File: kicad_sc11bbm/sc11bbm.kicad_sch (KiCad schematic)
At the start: 17 parts, among them M1 Brushless motor Right, M2 Brushless motor Left, Q1 2SK4017, U1 ESC_R, U2 ESC_L, U3 L3GD20H, U4 QMC5883L, U5 BMP280, U6 MW-R-DP-W, U7 AE-GYSFDMAXB, U8 ADXL335, U9 SD_CARD_DIP

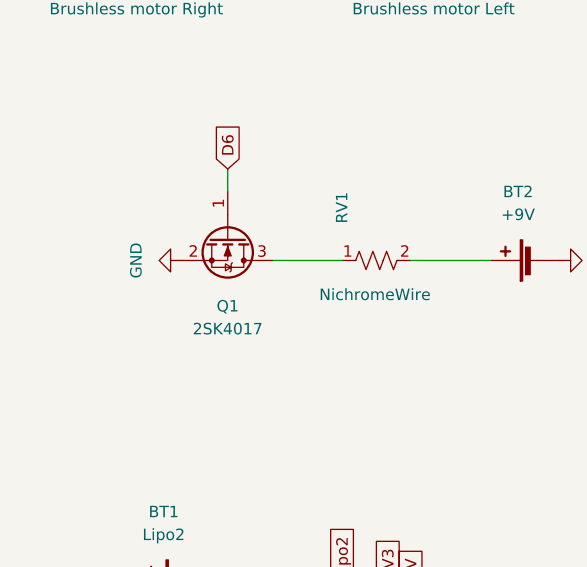
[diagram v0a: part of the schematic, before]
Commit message: Order completed for Board ver1.0
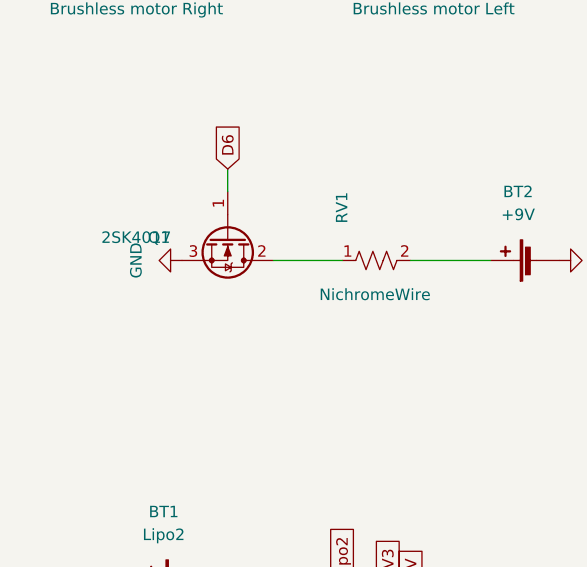
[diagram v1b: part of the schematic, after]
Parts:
- U3: footprint (none) -> sc11bbm:L3GD20H
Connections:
- net GND: now also Q1.3 (S); no longer Q1.2 (S)
- net at RV1.1: now also Q1.2 (D); no longer Q1.3 (D)
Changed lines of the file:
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@@
   (symbol (lib_id "Transistor_FET:2N7002E") (at 66.04 85.09 270) (unit 1)
     (in_bom yes) (on_board yes) (fields_autoplaced)
-    (property "Reference" "Q1" (id 0) (at 66.04 92.71 90))
-    (property "Value" "2SK4017" (id 1) (at 66.04 95.25 90))
-    (property "Footprint" "sc11bbm:2SK4017" (id 2) (at 64.135 90.17 0)
+    (property "Reference" "Q1" (id 0) (at 58.42 85.09 90))
+    (property "Value" "2SK4017" (id 1) (at 55.88 85.09 90))
+    (property "Footprint" "sc11bbm:2SK4017" (id 2) (at 60.96 83.185 0)
       (effects (font (size 1.27 1.27) italic) (justify left) hide)
     )
@@
     (property "Reference" "U3" (id 0) (at 199.39 111.76 0))
     (property "Value" "L3GD20H" (id 1) (at 199.39 114.3 0))
-    (property "Footprint" "" (id 2) (at 199.39 114.3 0)
+    (property "Footprint" "sc11bbm:L3GD20H" (id 2) (at 199.39 114.3 0)
       (effects (font (size 1.27 1.27)) hide)
     )
@@
     )
     (path "/bce30d9d-5959-43c2-901a-216240c51ddc"
-      (reference "U3") (unit 1) (value "L3GD20H") (footprint "")
+      (reference "U3") (unit 1) (value "L3GD20H") (footprint "sc11bbm:L3GD20H")
     )
     (path "/40d8ad8c-b3b9-4b74-ac6c-a025ffa51987"

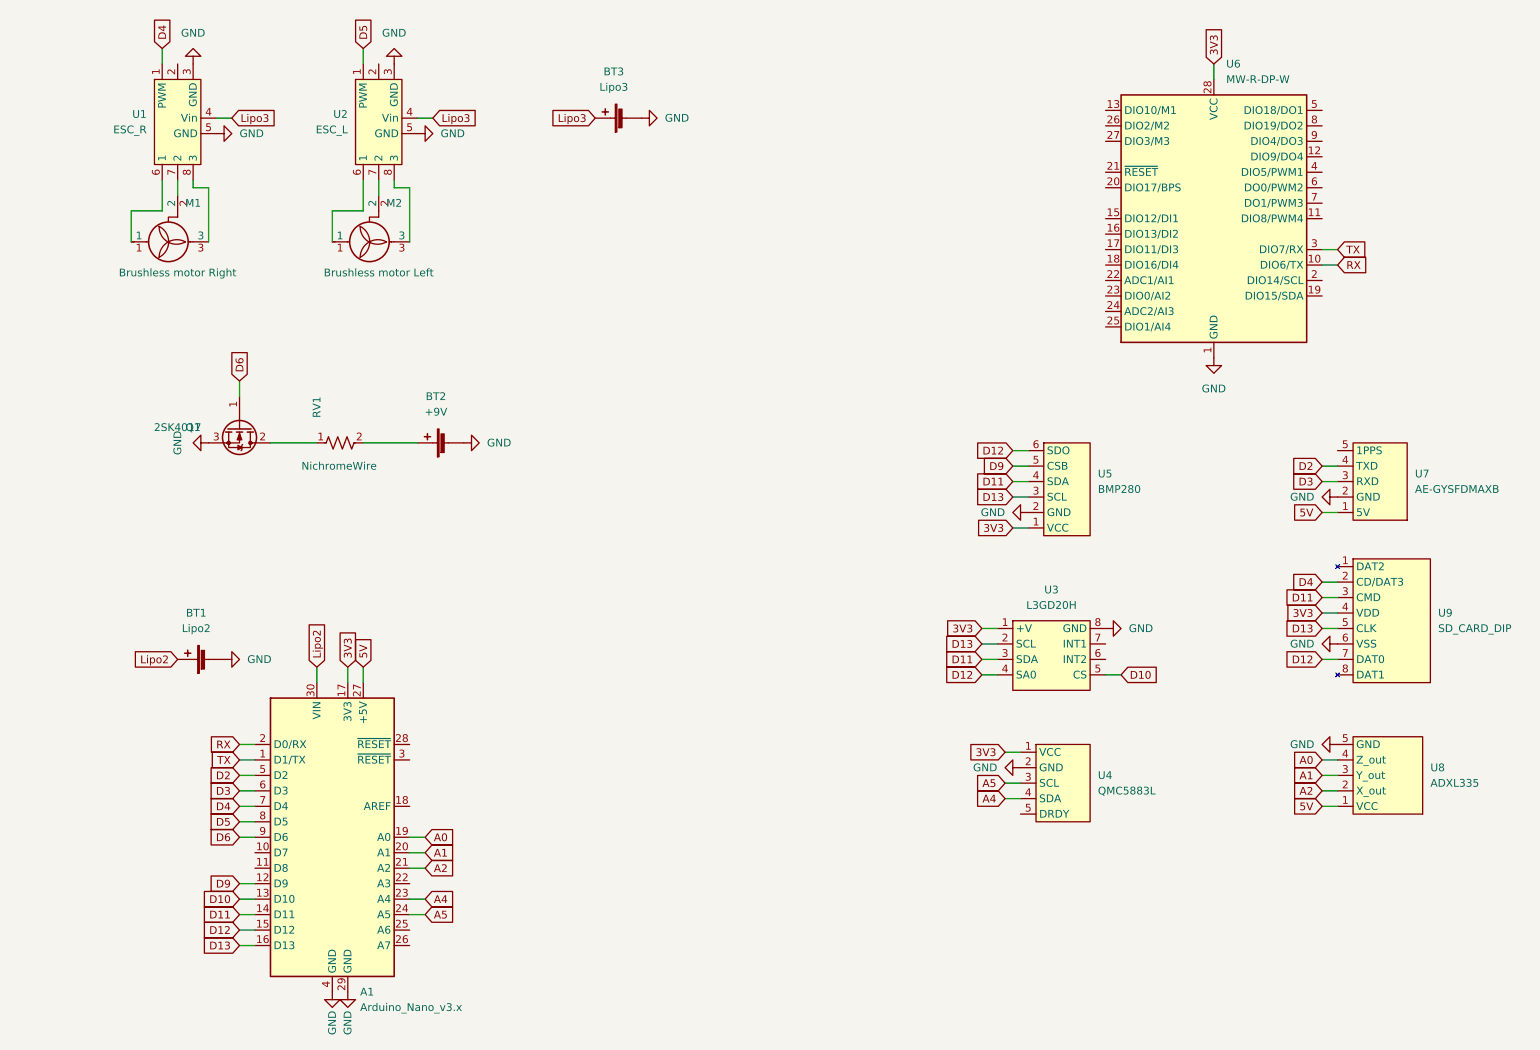
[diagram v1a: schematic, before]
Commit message: For EM board2
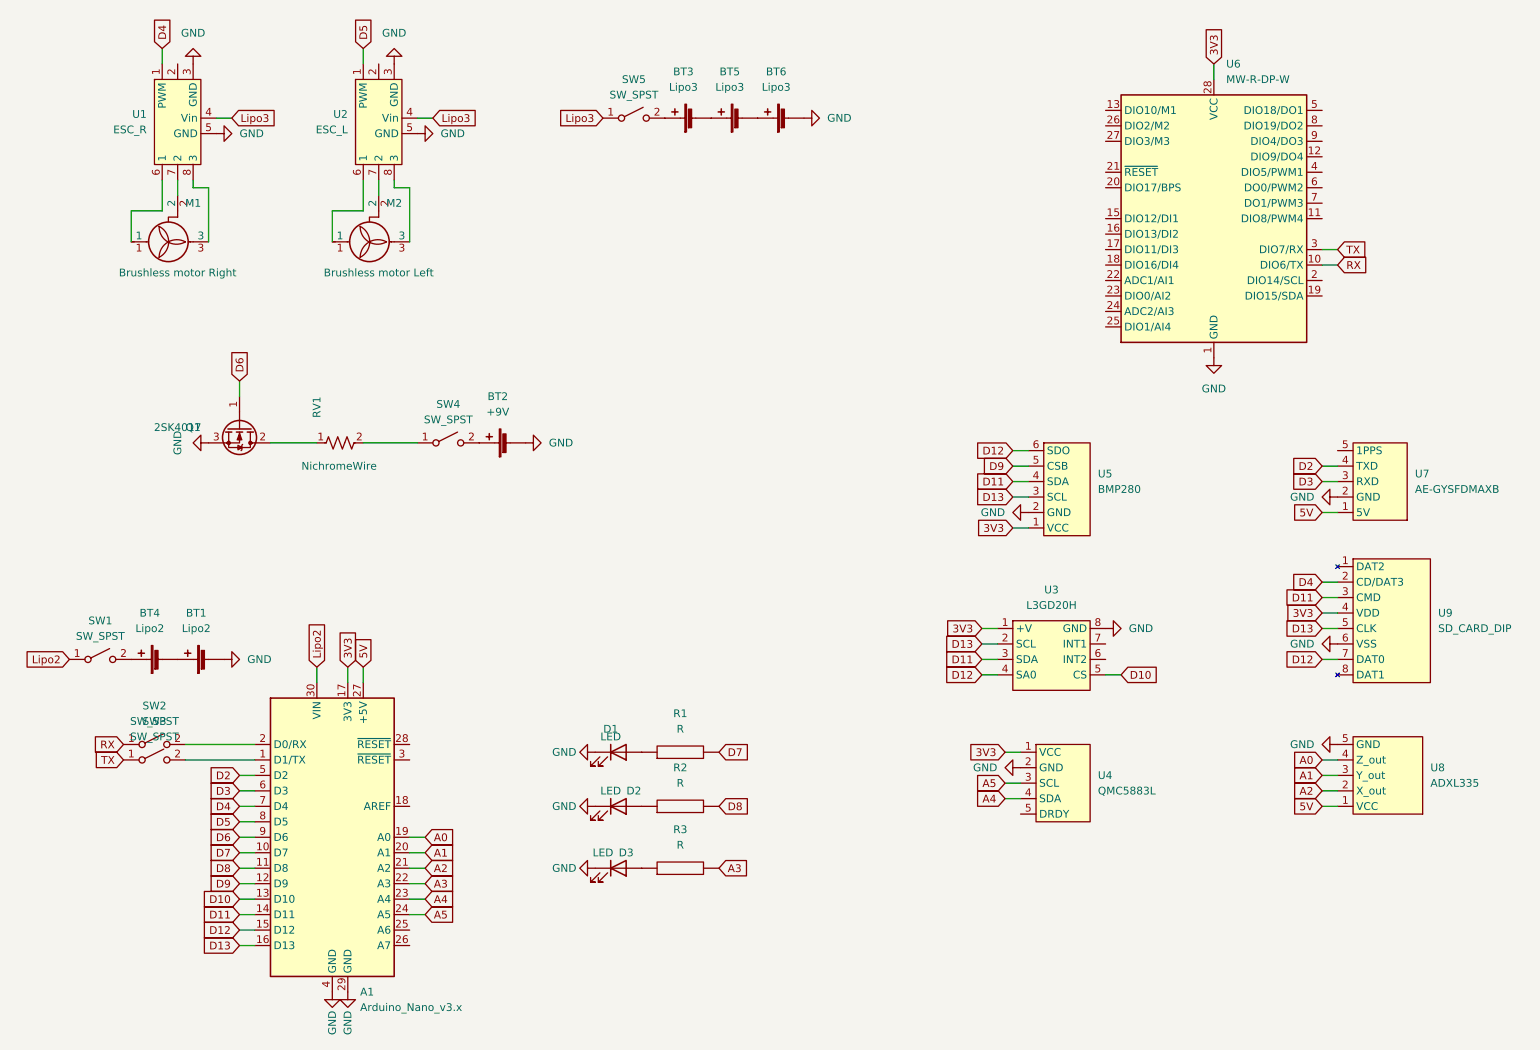
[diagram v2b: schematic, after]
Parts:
- added BT4: Lipo2, sc11bbm:Lipo2, symbol Device:Battery_Cell
- added BT5, BT6: Lipo3, sc11bbm:Lipo3, symbol Device:Battery_Cell
- added D1, D2, D3: LED, sc11bbm:LED, symbol Device:LED
- added R1, R2, R3: R, sc11bbm:Resistor, symbol pspice:R
- added SW1, SW2, SW3, SW4: SW_SPST, sc11bbm:swicth, symbol sc11bbm:SW_SPST
- added SW5: SW_SPST, sc11bbm:swicth, symbol Switch:SW_SPST
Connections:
- net GND: now also BT6.2 (-), D1.1 (K), D2.1 (K), D3.1 (K); no longer BT3.2 (-)
- net Lipo2: now also SW1.1 (A); no longer BT1.1 (+)
- net Lipo3: now also SW5.1 (A); no longer BT3.1 (+)
- net RX: now also SW2.1 (A); no longer A1.2 (D0/RX)
- net TX: now also SW3.1 (A); no longer A1.1 (D1/TX)
- net at RV1.2: now also SW4.1 (A); no longer BT2.1 (+)
- net D7: now reaches A1.10 (D7)
- net D7: now also R1.2
- net D8: now reaches A1.11 (D8)
- net D8: now also R2.2
- net A3: now reaches A1.22 (A3)
- net A3: now also R3.2
- new net: D1.2 (A), R1.1
- new net: BT3.2 (-), BT5.1 (+)
- new net: BT5.2 (-), BT6.1 (+)
- new net: D3.2 (A), R3.1
- new net: A1.1 (D1/TX), SW3.2 (B)
- new net: BT2.1 (+), SW4.2 (B)
- new net: BT3.1 (+), SW5.2 (B)
- new net: D2.2 (A), R2.1
- new net: BT4.1 (+), SW1.2 (B)
- new net: BT1.1 (+), BT4.2 (-)
- new net: A1.2 (D0/RX), SW2.2 (B)
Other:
- moved on the sheet: BT2, BT3
